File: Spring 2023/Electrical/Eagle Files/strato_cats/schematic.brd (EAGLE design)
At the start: 124.1 x 119.4 mm, 21 parts

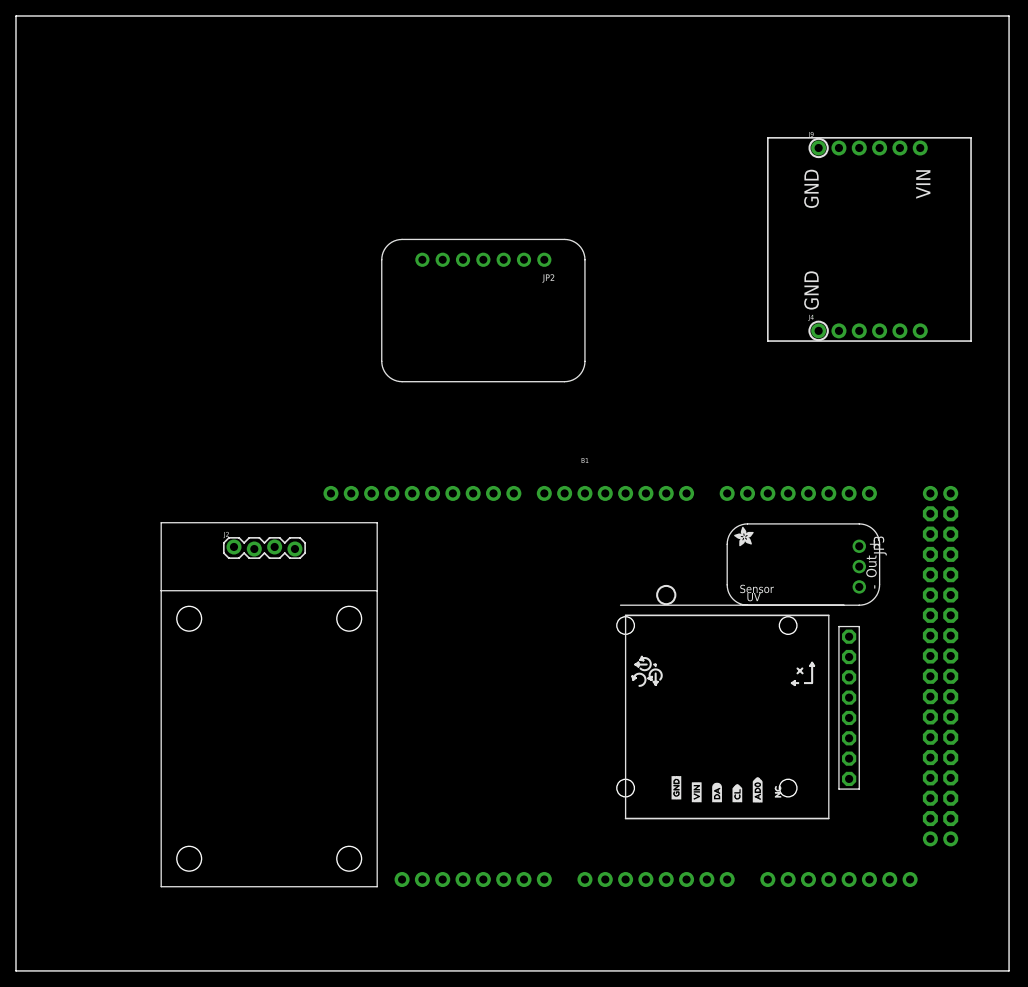
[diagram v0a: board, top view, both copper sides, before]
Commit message: finished board
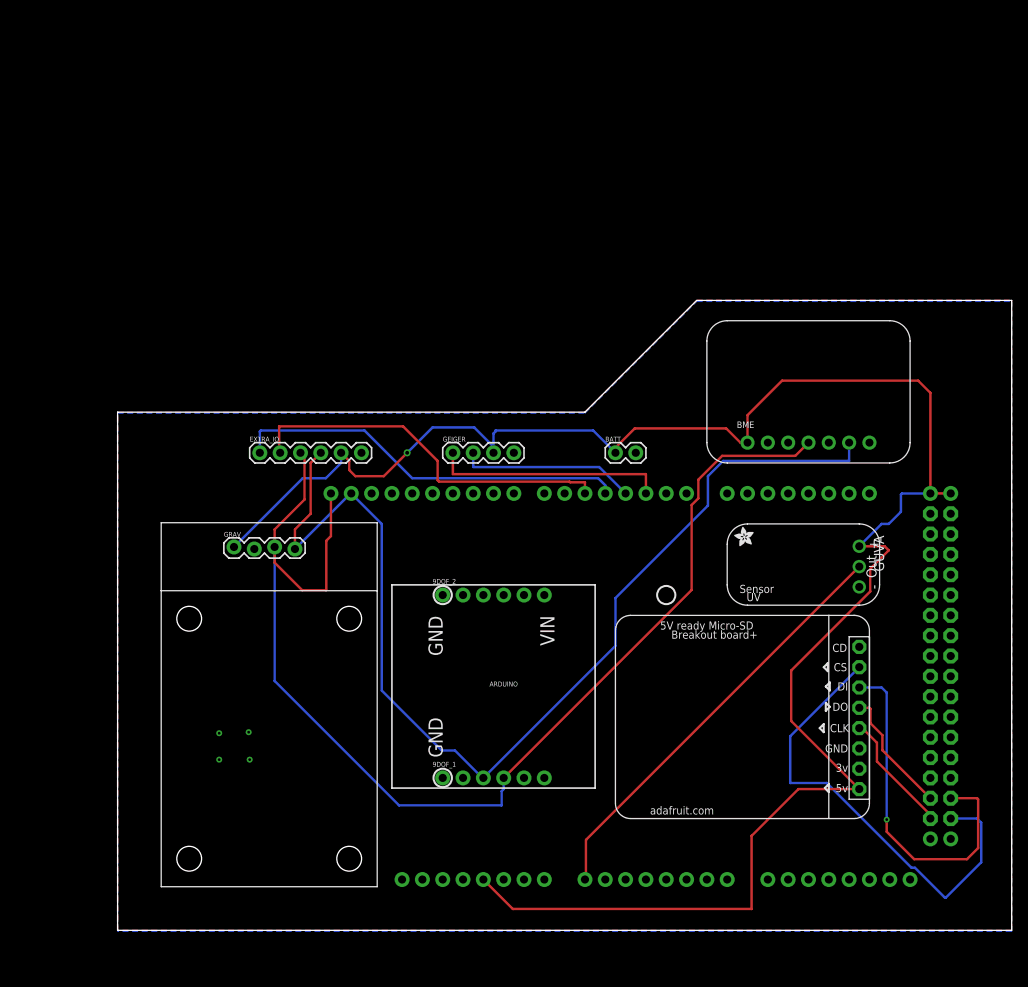
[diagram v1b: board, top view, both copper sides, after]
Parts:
- removed J4, J9: (no value), SparkFun-Connectors:1X06_NO_SILK
- removed JP2: (no value), microbuilder:1X07_ROUND_70
- removed JP4: (no value), adafruit:1X08-BIG
- removed U$47, U$74: (no value), buzzard_labels_2:GND4
- removed U$62: (no value), buzzard_labels_2:MISO13
- removed U$63: (no value), buzzard_labels_2:MOSI14
- removed U$64: (no value), buzzard_labels_2:SCLK15
- removed U$65: (no value), buzzard_labels_2:#CS16
- removed U$66: (no value), buzzard_labels_2:1V8#5V57
- removed U$67: (no value), buzzard_labels_2:VIN5
- removed U$68: (no value), buzzard_labels_2:NC17
- removed U$69: (no value), buzzard_labels_2:AD012
- removed U$89: (no value), buzzard_labels:CL4
- removed U$90: (no value), buzzard_labels:DA2
- added 9DOF_1, 9DOF_2: (no value), SparkFun-Connectors:1X06_NO_SILK
- added BATT: (no value), SparkFun-Connectors:1X02
- added BME: (no value), microbuilder:1X07_ROUND_70
- added EXTRA_IO: (no value), SparkFun-Connectors:1X06
- added GEIGER: (no value), SparkFun-Connectors:1X04
- added SD_R: (no value), adafruit:1X08-BIG
- renumbered B1 to ARDUINO, J2 to GRAV, JP3 to GUVA
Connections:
- removed net !CS!_VIN: ARDUINO.7, J4.6
- removed net +3V3: JP4.2
- removed net 5V*3: ARDUINO.5V, ARDUINO.5V@1, ARDUINO.5V@2, GRAV.1, GUVA.1, J4.2, J9.6, JP2.1, JP4.1
- removed net AD0/SDO_VIN: J4.5
- removed net AUX_CL_VIN: J9.5
- removed net AUX_DA_VIN: J9.4
- removed net CD: JP4.8
- removed net DI: ARDUINO.51, JP4.6
- removed net DO: ARDUINO.50, JP4.5
- removed net FSYNC_VIN: J9.3
- removed net INT_VIN: J9.2
- removed net N$2: JP2.2
- removed net SDA/SDI_VIN: ARDUINO.20, GRAV.4, J4.3, JP2.6
- removed net SDO/ADR: JP2.5
- new net 3V: 9DOF_1.2
- new net 5V: ARDUINO.5V, ARDUINO.5V@1, ARDUINO.5V@2, BATT.1, BME.1, EXTRA_IO.5, GEIGER.3, GRAV.1, GUVA.1, SD_R.1
- new net D4: ARDUINO.4, EXTRA_IO.1
- new net D5: ARDUINO.5, EXTRA_IO.2
- new net DS: ARDUINO.3, GEIGER.2
- new net NS: ARDUINO.2, GEIGER.1
- new net SDA: 9DOF_1.3, ARDUINO.SDA, BME.6, EXTRA_IO.4, GRAV.4
- new net SDI: ARDUINO.51, SD_R.6
- new net SDO: ARDUINO.50, SD_R.5
- net CLK: now also SD_R.4; no longer JP4.4
- net CS: now also SD_R.7; no longer JP2.7, JP4.7
- net GND: now also 9DOF_1.1, 9DOF_2.1, ARDUINO.GND@1, ARDUINO.GND@2, BATT.2, BME.3, EXTRA_IO.6, GEIGER.4, SD_R.3; no longer J4.1, J9.1, JP2.3, JP4.3
- net SCL: now also 9DOF_1.4, ARDUINO.SCL, BME.4, EXTRA_IO.3; no longer ARDUINO.21, J4.4, JP2.4
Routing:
- net 5V: track 0.00 -> 241.3 mm, vias 0 -> 1
- net SCL: track 0.00 -> 153.9 mm
- net SDA: track 0.00 -> 136.8 mm
- net CS: track 0.00 -> 58.7 mm
- net N$1: track 0.00 -> 53.3 mm
- net D4: track 0.00 -> 49.8 mm
- net D5: track 0.00 -> 47.3 mm
- net SDI: track 0.00 -> 44.1 mm, vias 0 -> 1
- net NS: track 0.00 -> 29.2 mm
- net DS: track 0.00 -> 22.2 mm
- net SDO: track 0.00 -> 15.7 mm
- net CLK: track 0.00 -> 15.2 mm
- added copper zone on layer 1, net GND
- added copper zone on layer 16, net GND
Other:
- board size 124.1 x 119.4 mm -> 111.8 x 78.7 mm
- board text added: "3v"
- board text added: "5V ready Micro-SD"
- board text added: "5v"
- board text added: "Breakout board+"
- board text added: "CD"
- board text added: "CLK"
- board text added: "CS"
- board text added: "DI"
- board text added: "DO"
- board text added: "adafruit.com"
- board text removed: "Owen Lyke"
